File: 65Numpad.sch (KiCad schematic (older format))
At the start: 41 parts

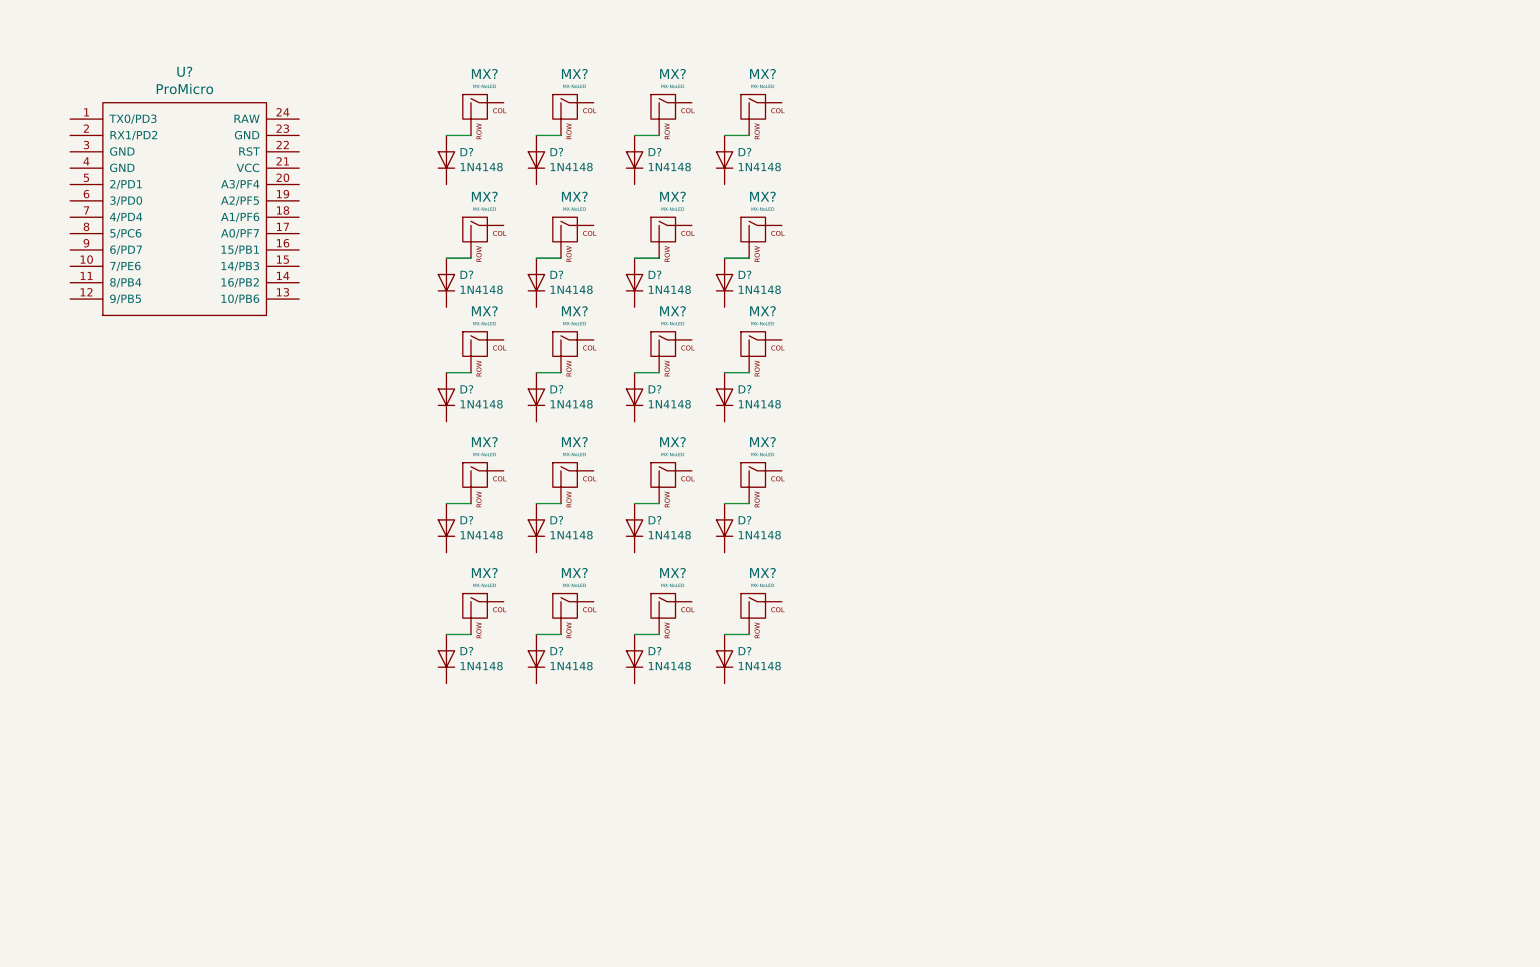
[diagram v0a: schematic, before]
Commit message: Matrix setup
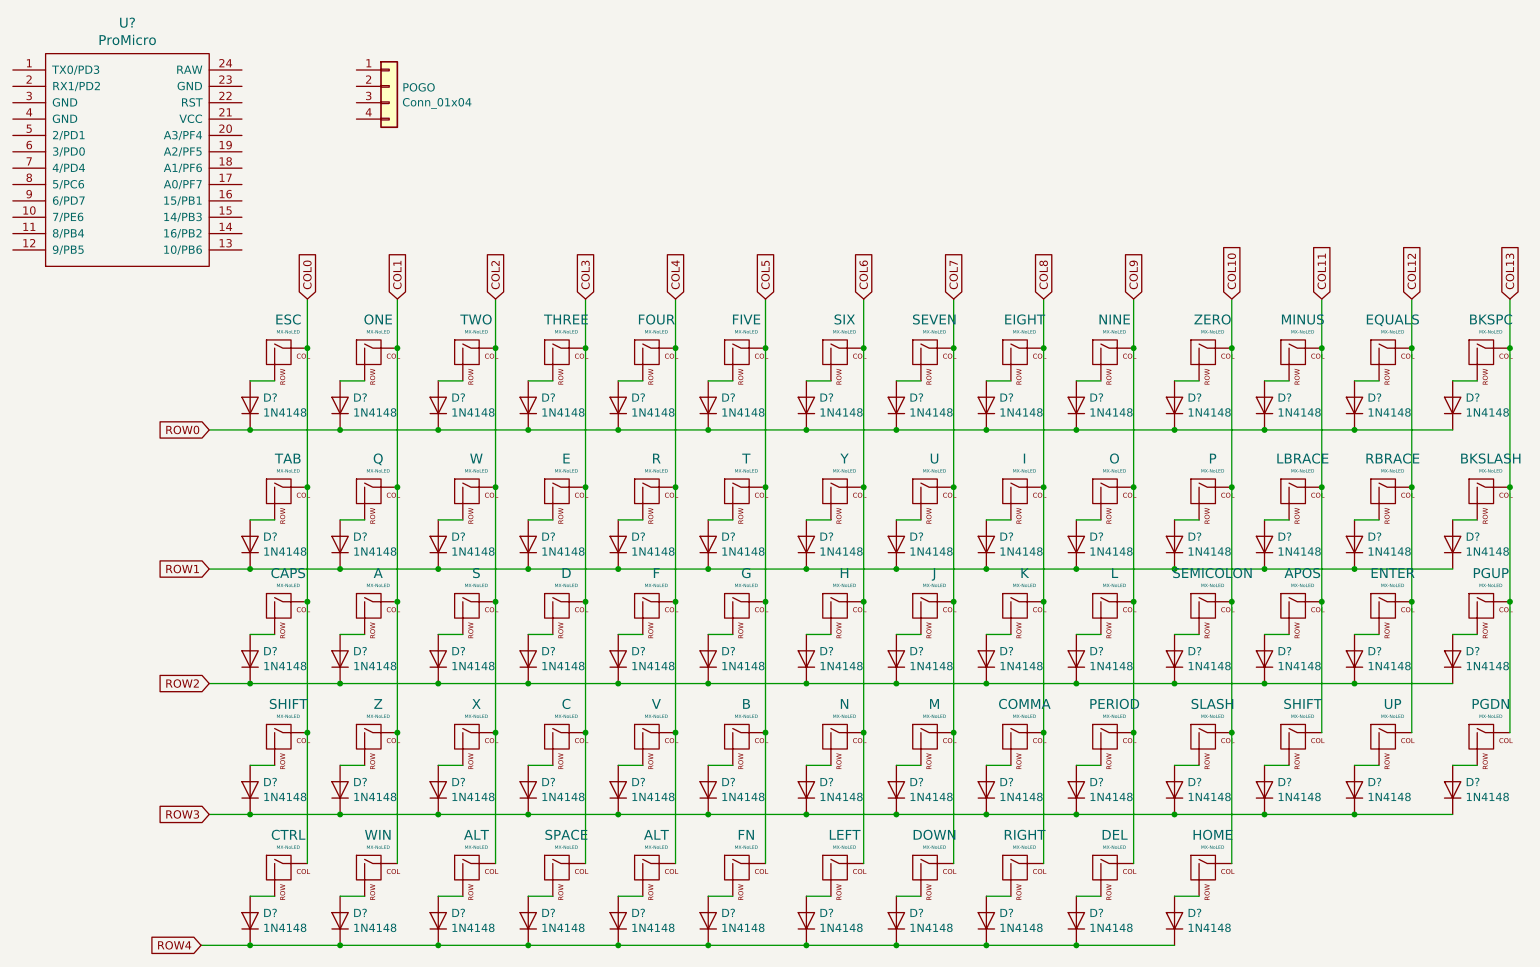
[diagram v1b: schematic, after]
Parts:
- added ALT, APOS, B, BKSLASH, BKSPC, COMMA, DEL, DOWN, EIGHT, ENTER, EQUALS, F, FIVE, FN, FOUR, G, H, HOME, I, J, K, L, LBRACE, LEFT, M, MINUS, N, NINE, O, P, PERIOD, PGDN, PGUP, R, RBRACE, RIGHT, SEMICOLON, SEVEN, SHIFT, SIX, SLASH, T, U, UP, V, Y, ZERO: MX-NoLED, symbol MX_Alps_Hybrid:MX-NoLED
- added D? (x47): 1N4148, Diode_THT:D_DO-35_SOD27_P7.62mm_Horizontal, symbol Diode:1N4148
- added POGO: Conn_01x04, symbol Connector_Generic:Conn_01x04
- gave numbers to parts that had none: 20
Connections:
- net COL0: now reaches ESC.1 (COL)
- net COL0: now also CAPS.1 (COL), CTRL.1 (COL), SHIFT.1 (COL), TAB.1 (COL)
- net ROW0: now reaches D?.1 (K)
- net ROW0: now also D?.1 (K), D?.1 (K), D?.1 (K), D?.1 (K), D?.1 (K), D?.1 (K), D?.1 (K), D?.1 (K), D?.1 (K), D?.1 (K), D?.1 (K), D?.1 (K), D?.1 (K)
- net COL1: now reaches ONE.1 (COL)
- net COL1: now also A.1 (COL), Q.1 (COL), WIN.1 (COL), Z.1 (COL)
- net COL2: now reaches TWO.1 (COL)
- net COL2: now also ALT.1 (COL), S.1 (COL), W.1 (COL), X.1 (COL)
- net COL3: now reaches THREE.1 (COL)
- net COL3: now also C.1 (COL), D.1 (COL), E.1 (COL), SPACE.1 (COL)
- net ROW1: now reaches D?.1 (K)
- net ROW1: now also D?.1 (K), D?.1 (K), D?.1 (K), D?.1 (K), D?.1 (K), D?.1 (K), D?.1 (K), D?.1 (K), D?.1 (K), D?.1 (K), D?.1 (K), D?.1 (K), D?.1 (K)
- net ROW2: now reaches D?.1 (K)
- net ROW2: now also D?.1 (K), D?.1 (K), D?.1 (K), D?.1 (K), D?.1 (K), D?.1 (K), D?.1 (K), D?.1 (K), D?.1 (K), D?.1 (K), D?.1 (K), D?.1 (K), D?.1 (K)
- net ROW3: now reaches D?.1 (K)
- net ROW3: now also D?.1 (K), D?.1 (K), D?.1 (K), D?.1 (K), D?.1 (K), D?.1 (K), D?.1 (K), D?.1 (K), D?.1 (K), D?.1 (K), D?.1 (K), D?.1 (K), D?.1 (K)
- net ROW4: now reaches D?.1 (K)
- net ROW4: now also D?.1 (K), D?.1 (K), D?.1 (K), D?.1 (K), D?.1 (K), D?.1 (K), D?.1 (K), D?.1 (K), D?.1 (K), D?.1 (K)
- new net: D?.2 (A), FOUR.2 (ROW)
- new net: D?.2 (A), FIVE.2 (ROW)
- new net: D?.2 (A), SIX.2 (ROW)
- new net: D?.2 (A), SEVEN.2 (ROW)
- new net: D?.2 (A), R.2 (ROW)
- new net: D?.2 (A), T.2 (ROW)
- new net: D?.2 (A), Y.2 (ROW)
- new net: D?.2 (A), U.2 (ROW)
- new net: D?.2 (A), F.2 (ROW)
- new net: D?.2 (A), G.2 (ROW)
- new net: D?.2 (A), H.2 (ROW)
- new net: D?.2 (A), J.2 (ROW)
- new net: D?.2 (A), V.2 (ROW)
- new net: B.2 (ROW), D?.2 (A)
- new net: D?.2 (A), N.2 (ROW)
- new net: D?.2 (A), M.2 (ROW)
- new net: ALT.2 (ROW), D?.2 (A)
- new net: D?.2 (A), FN.2 (ROW)
- new net: D?.2 (A), LEFT.2 (ROW)
- new net: D?.2 (A), DOWN.2 (ROW)
- new net: D?.2 (A), EIGHT.2 (ROW)
- new net: D?.2 (A), NINE.2 (ROW)
- new net: D?.2 (A), ZERO.2 (ROW)
- new net: D?.2 (A), MINUS.2 (ROW)
- new net: D?.2 (A), I.2 (ROW)
- new net: D?.2 (A), O.2 (ROW)
- new net: D?.2 (A), P.2 (ROW)
- new net: D?.2 (A), LBRACE.2 (ROW)
- new net: D?.2 (A), K.2 (ROW)
- new net: D?.2 (A), L.2 (ROW)
- new net: D?.2 (A), SEMICOLON.2 (ROW)
- new net: APOS.2 (ROW), D?.2 (A)
- new net: COMMA.2 (ROW), D?.2 (A)
- new net: D?.2 (A), PERIOD.2 (ROW)
- new net: D?.2 (A), SLASH.2 (ROW)
- new net: D?.2 (A), SHIFT.2 (ROW)
- new net: D?.2 (A), RIGHT.2 (ROW)
- new net: D?.2 (A), EQUALS.2 (ROW)
- new net: BKSPC.2 (ROW), D?.2 (A)
- new net: D?.2 (A), DEL.2 (ROW)
- new net: D?.2 (A), RBRACE.2 (ROW)
- new net: BKSLASH.2 (ROW), D?.2 (A)
- new net: D?.2 (A), HOME.2 (ROW)
- new net: D?.2 (A), ENTER.2 (ROW)
- new net: D?.2 (A), PGUP.2 (ROW)
- new net: D?.2 (A), UP.2 (ROW)
- new net: D?.2 (A), PGDN.2 (ROW)
- new net COL10: HOME.1 (COL), P.1 (COL), SEMICOLON.1 (COL), SLASH.1 (COL), ZERO.1 (COL)
- new net COL11: APOS.1 (COL), LBRACE.1 (COL), MINUS.1 (COL), SHIFT.1 (COL)
- new net COL12: ENTER.1 (COL), EQUALS.1 (COL), RBRACE.1 (COL), UP.1 (COL)
- new net COL13: BKSLASH.1 (COL), BKSPC.1 (COL), PGDN.1 (COL), PGUP.1 (COL)
- new net COL4: ALT.1 (COL), F.1 (COL), FOUR.1 (COL), R.1 (COL), V.1 (COL)
- new net COL5: B.1 (COL), FIVE.1 (COL), FN.1 (COL), G.1 (COL), T.1 (COL)
- new net COL6: H.1 (COL), LEFT.1 (COL), N.1 (COL), SIX.1 (COL), Y.1 (COL)
- new net COL7: DOWN.1 (COL), J.1 (COL), M.1 (COL), SEVEN.1 (COL), U.1 (COL)
- new net COL8: COMMA.1 (COL), EIGHT.1 (COL), I.1 (COL), K.1 (COL), RIGHT.1 (COL)
- new net COL9: DEL.1 (COL), L.1 (COL), NINE.1 (COL), O.1 (COL), PERIOD.1 (COL)
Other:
- moved on the sheet: A, ALT, C, CAPS, CTRL, D, D?, E, ESC, ONE, Q, S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
